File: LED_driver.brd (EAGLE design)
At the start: 100 x 80 mm, 15 parts

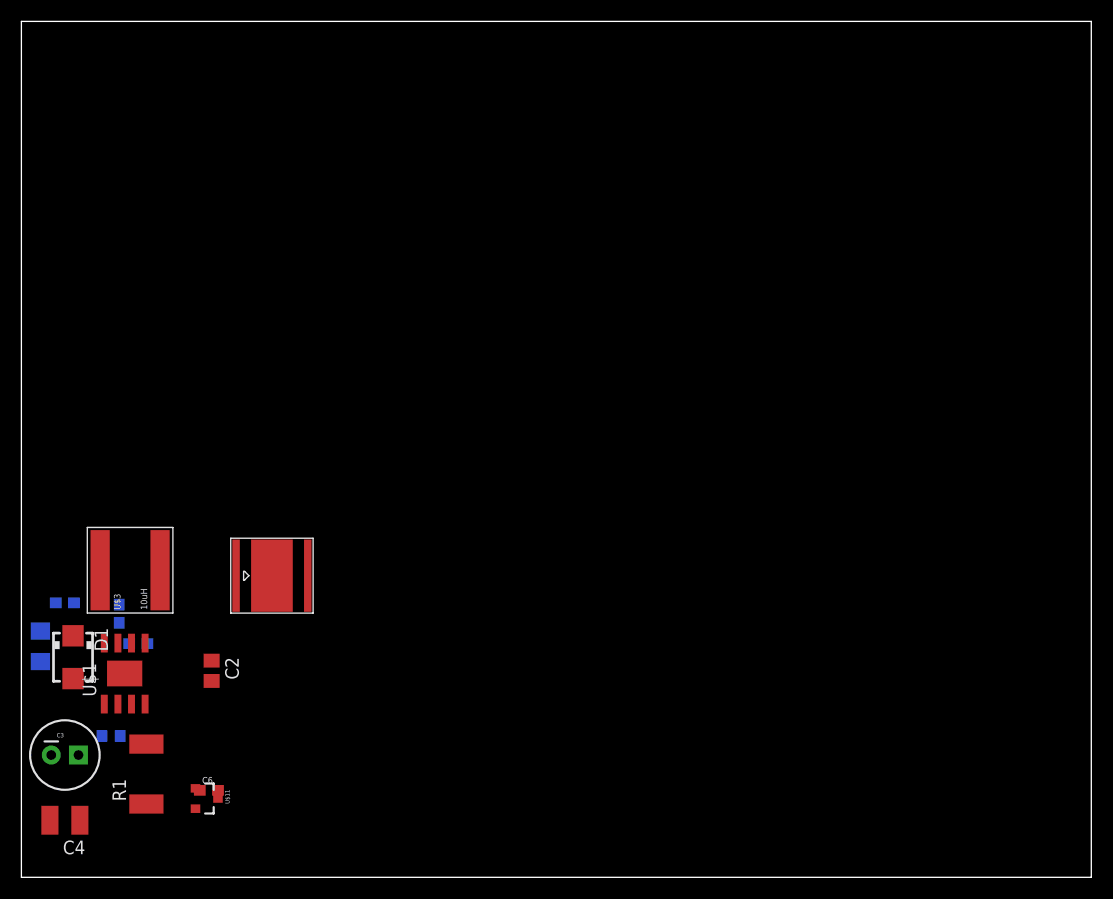
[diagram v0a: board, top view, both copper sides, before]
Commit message: Almost done with version 1 of the LED Driver Board
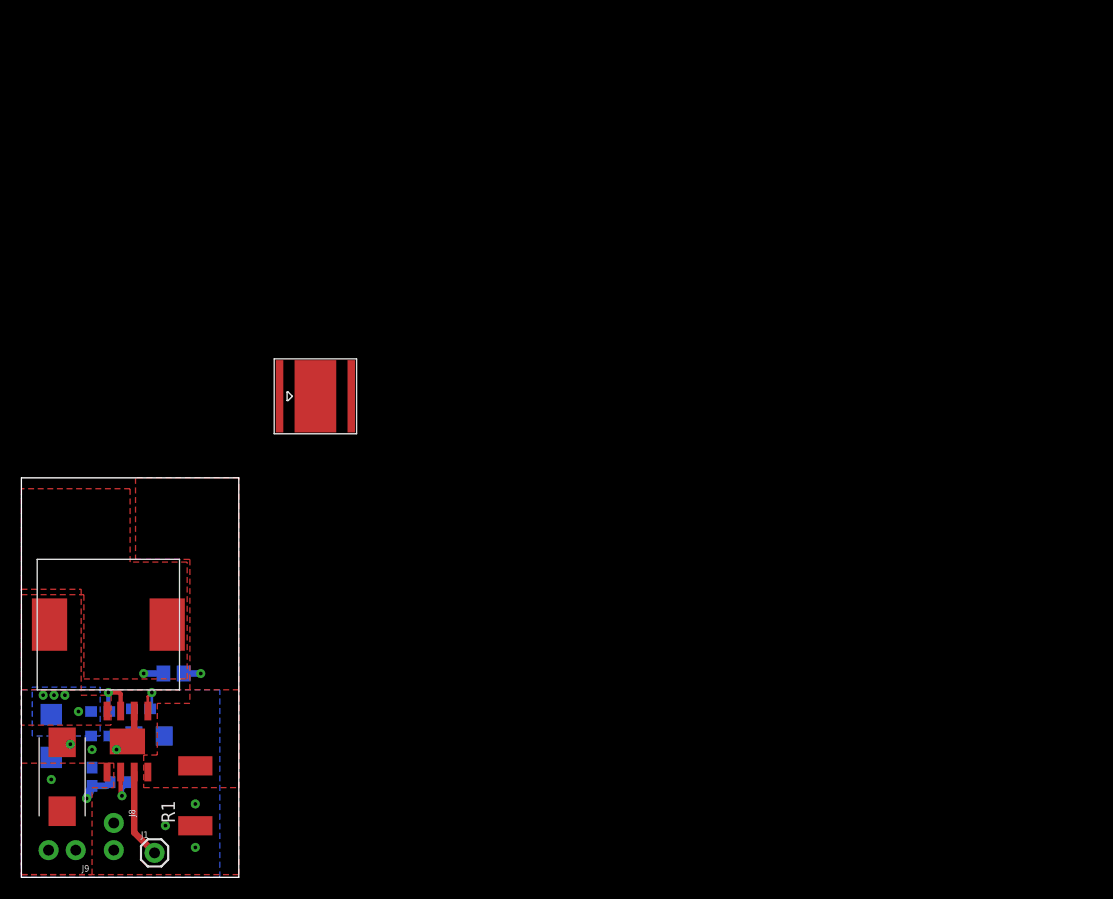
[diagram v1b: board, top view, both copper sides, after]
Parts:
- removed C4: 4.7uF 80V, resistor:C1210
- removed C6: 10uF, resistor:C0603
- removed U$11: VREG-ZXTR2105, BlueRobotics-Main:SOT23-3
- removed U$3: 10uH, BlueRobotics-Main:INDUCTOR-8040
- added C8: 47uF, PowerComponents:CTAN(7.30_4.30MM)
- added J1: (no value), SparkFun-Connectors:1X01
- added J8, J9: (no value), SparkFun-Connectors:1X02_NO_SILK
- added U$4: 15uH, DiscreteComponents:HCMA1305
- C3: value 47uF 63V -> 4.7uF; device SparkFun-Capacitors:CPOL-RADIAL-100UF-25V -> rcl:C0603
- moved U$2 17.2 mm to (24.1, 45.0)
- moved R7 13.2 mm to (11.9, 13.2), turned to 180 degrees
- moved C7 12.9 mm to (7.37, 13.2), turned to 180 degrees
- moved C5 9.32 mm to (7.37, 15.5), turned to 180 degrees
- moved D1 7.64 mm to (2.79, 13.2), flipped to the bottom
- moved U$1 6.36 mm to (9.91, 12.7)
- moved C1 6.10 mm to (11.2, 15.7)
- moved R1 5.00 mm to (16.3, 7.62)
- moved R2 4.38 mm to (9.14, 8.89)
- moved C2 3.57 mm to (14.2, 19.1), flipped to the bottom, turned to 180 degrees
- moved C3 3.25 mm to (6.60, 9.40), flipped to the bottom, turned to 90 degrees
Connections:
- removed net VCC: C6.1, U$11.2
- net GND: now also C8.-, J8.1, J8.2; no longer C4.2, C6.2, U$11.1
- net LED+: now also U$4.P$2; no longer U$3.P$2
- net LED-PWM: now also J1.1
- net N$5: now also U$4.P$1; no longer U$3.P$1
- net VIN: now also C8.+, J9.1, J9.2; no longer C4.1, U$11.3
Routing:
- net LED-PWM: track 0.00 -> 8.34 mm
- net N$4: track 0.00 -> 4.62 mm, vias 0 -> 1
- net GND: track 0.00 -> 3.94 mm, vias 0 -> 7
- net N$1: track 0.00 -> 3.79 mm, vias 0 -> 1
- net VCC6211: track 0.00 -> 3.48 mm, vias 0 -> 1
- net VIN: track 0.00 -> 3.12 mm, vias 0 -> 1
- net N$2: track 0.00 -> 2.30 mm
- net LED+: track 0.00 -> 1.84 mm, vias 0 -> 1
- net LED-: track 0.00 -> 1.59 mm, vias 0 -> 1
- added copper zone on layer 1, net GND
- added copper zone on layer 16, net GND
- added copper zone on layer 1, net LED+
- added copper zone on layer 1, net LED-
- added copper zone on layer 1, net N$5
- added copper zone on layer 16, net N$5
- added copper zone on layer 1, net VIN
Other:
- board size 100 x 80 mm -> 20.3 x 37.3 mm
